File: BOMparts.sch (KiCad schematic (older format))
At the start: 12 parts

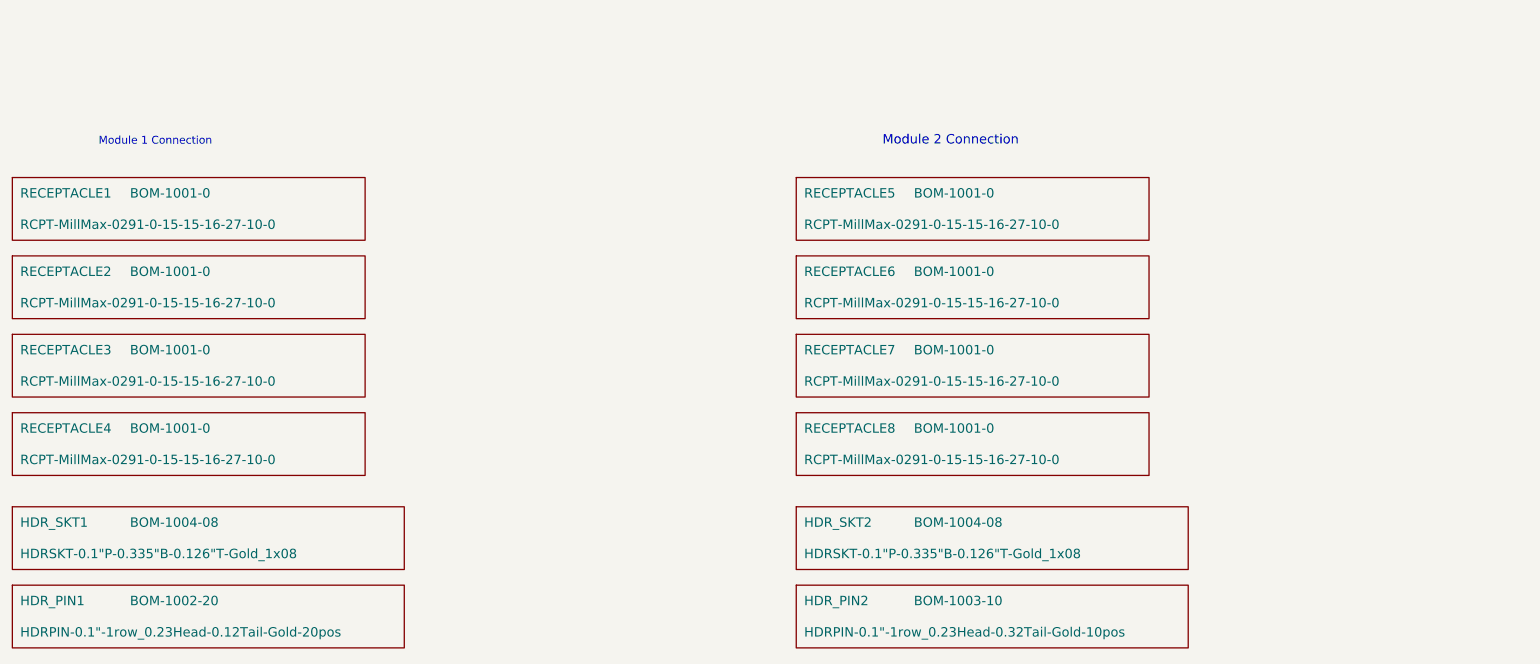
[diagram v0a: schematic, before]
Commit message: Rev 2 Schematic
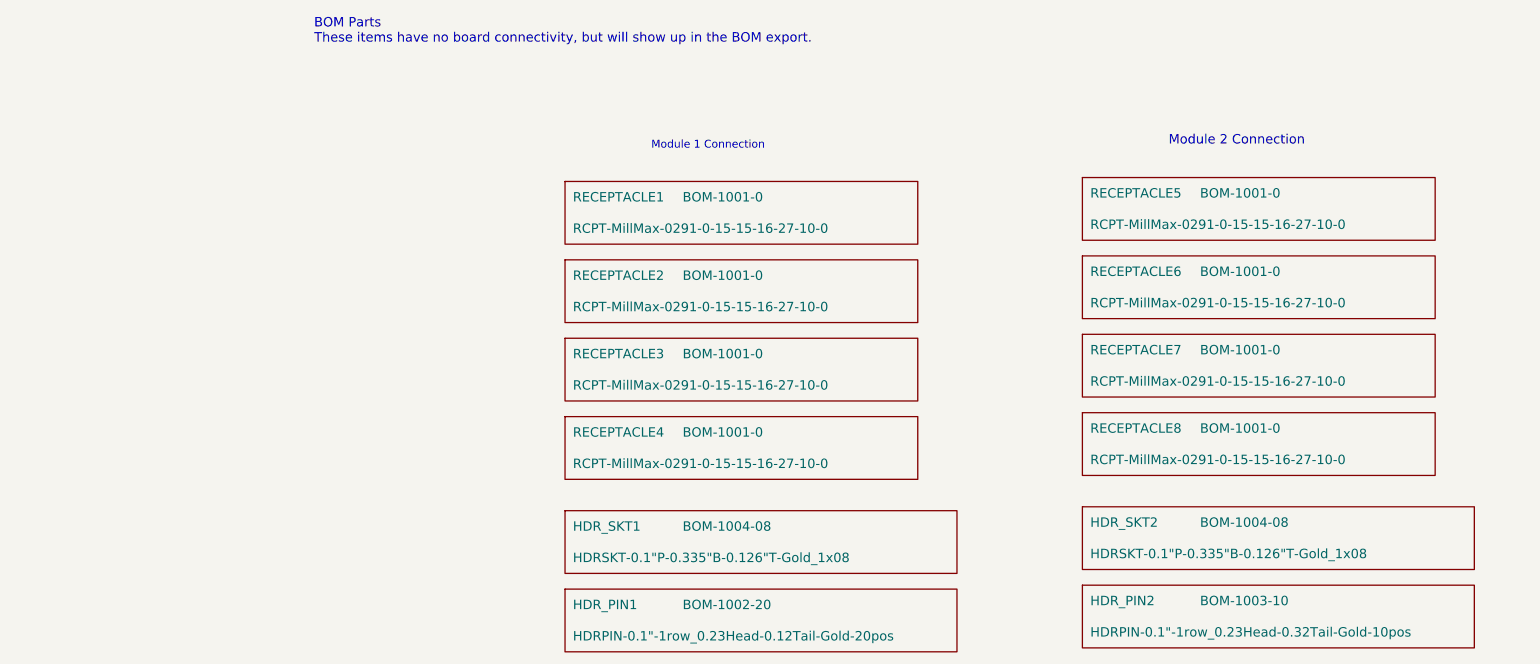
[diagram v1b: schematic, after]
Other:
- note added: "BOM Parts\nThese items have no board connectivity, but will show up in the BOM export."
- moved on the sheet: HDR_PIN1, HDR_PIN2, HDR_SKT1, HDR_SKT2, RECEPTACLE1, RECEPTACLE2, RECEPTACLE3, RECEPTACLE4, RECEPTACLE5, RECEPTACLE6, RECEPTACLE7, RECEPTACLE8
